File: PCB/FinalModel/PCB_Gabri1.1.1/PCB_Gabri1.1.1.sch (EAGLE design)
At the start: 5 parts, among them U3 TXS0104ED, X1 0446200002

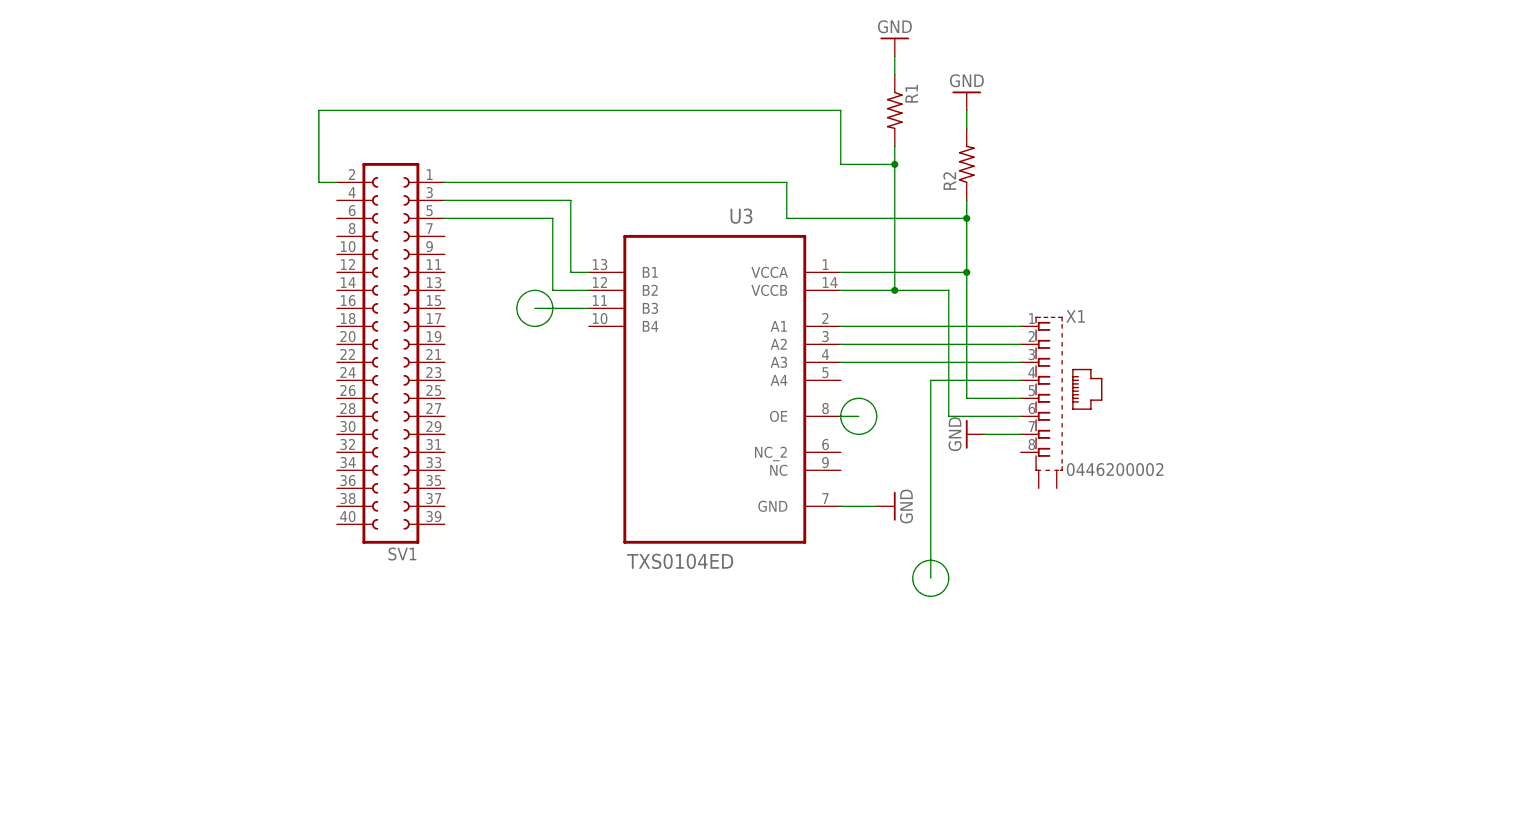
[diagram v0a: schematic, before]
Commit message: LAB 06022019
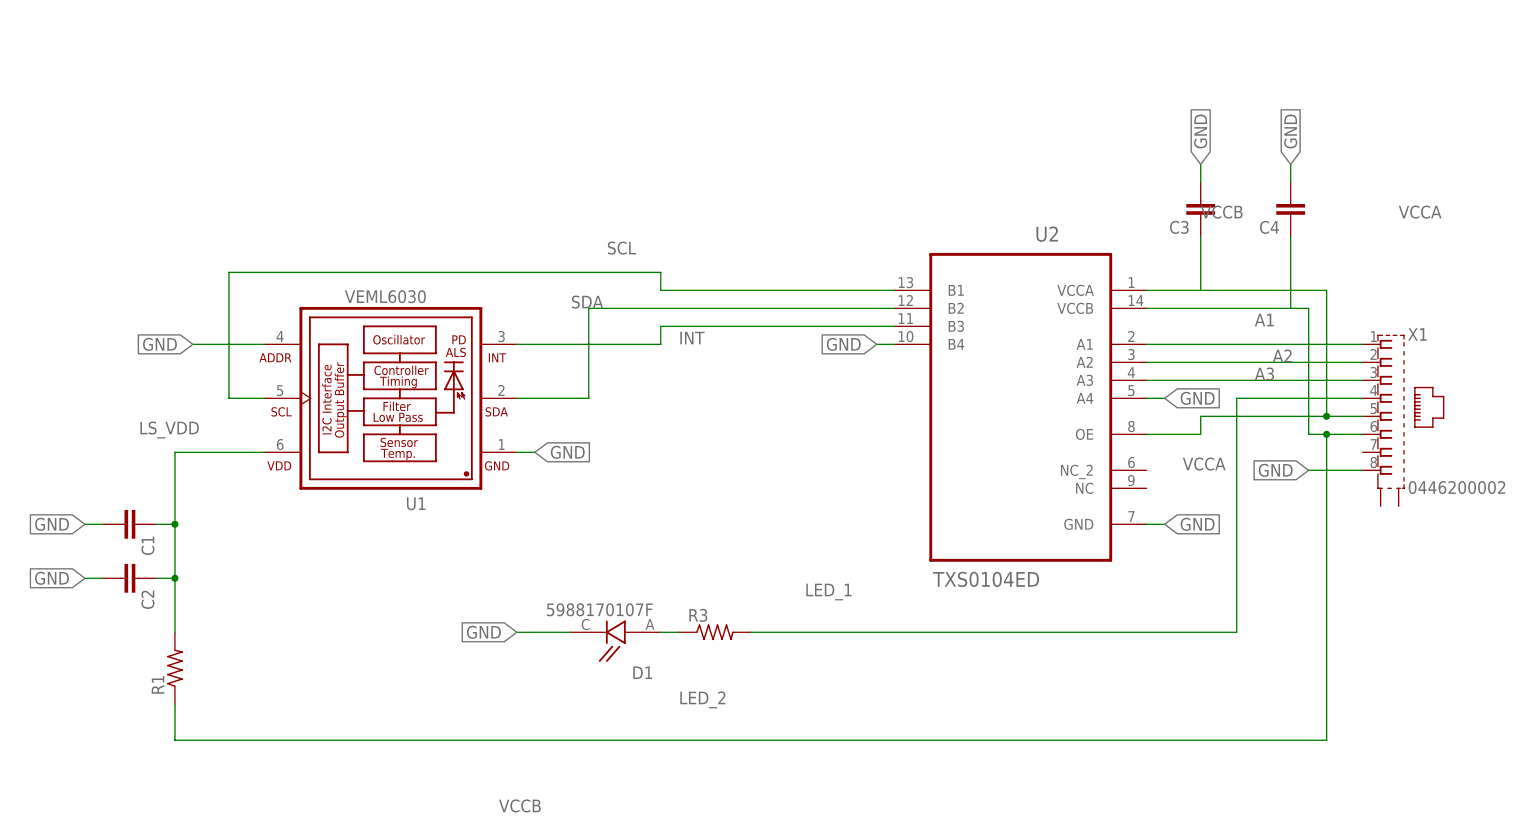
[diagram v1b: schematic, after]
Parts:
- removed R2: (no value), resistor:R-US_R0805
- removed SV1: (no value), con-lsta:FE20-2
- removed U3: TXS0104ED, TXS0104ED:TXS0104ED
- added C1, C2, C3, C4: (no value), resistor:C-EU025-024X044
- added D1: 5988170107F, 5988170107F:5988170107F
- added R3: (no value), resistor:R-US_R0805
- added U1: VEML6030, VEML6030:VEML6030
- added U2: TXS0104ED, TXS0104ED:TXS0104ED
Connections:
- removed net N$1: U3.A1, X1.1
- removed net N$10: X1.4
- removed net N$2: U3.A2, X1.2
- removed net N$3: U3.A3, X1.3
- removed net N$4: R2.1, SV1.1, U3.VCCA, X1.5
- removed net N$5: R1.2, SV1.2, U3.VCCB, X1.6
- removed net N$6: SV1.3, U3.B1
- removed net N$7: SV1.5, U3.B2
- removed net N$8: U3.B3
- removed net N$9: U3.OE
- new net A1: U2.A1, X1.1
- new net A2: U2.A2, X1.2
- new net A3: U2.A3, X1.3
- new net INT: U1.INT, U2.B3
- new net LED_1: R3.2, X1.4
- new net LED_2: D1.A, R3.1
- new net LS_VDD: C1.1, C2.1, R1.2, U1.VDD
- new net SCL: U1.SCL, U2.B1
- new net SDA: U1.SDA, U2.B2
- new net VCCA: C3.1, U2.OE, U2.VCCA, X1.5
- new net VCCB: C4.1, R1.1, U2.VCCB, X1.6
- net GND: now also C1.2, C2.2, C3.2, C4.2, D1.C, U1.ADDR, U1.GND, U2.A4, U2.B4, U2.GND, X1.8; no longer R1.1, R2.2, U3.GND, X1.7
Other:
- moved on the sheet: R1, X1
